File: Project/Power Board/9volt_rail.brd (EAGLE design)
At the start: 98.3 x 69.5 mm, 54 parts, among them IC1 TL331, Q1 BSS84, Q2 BSS123

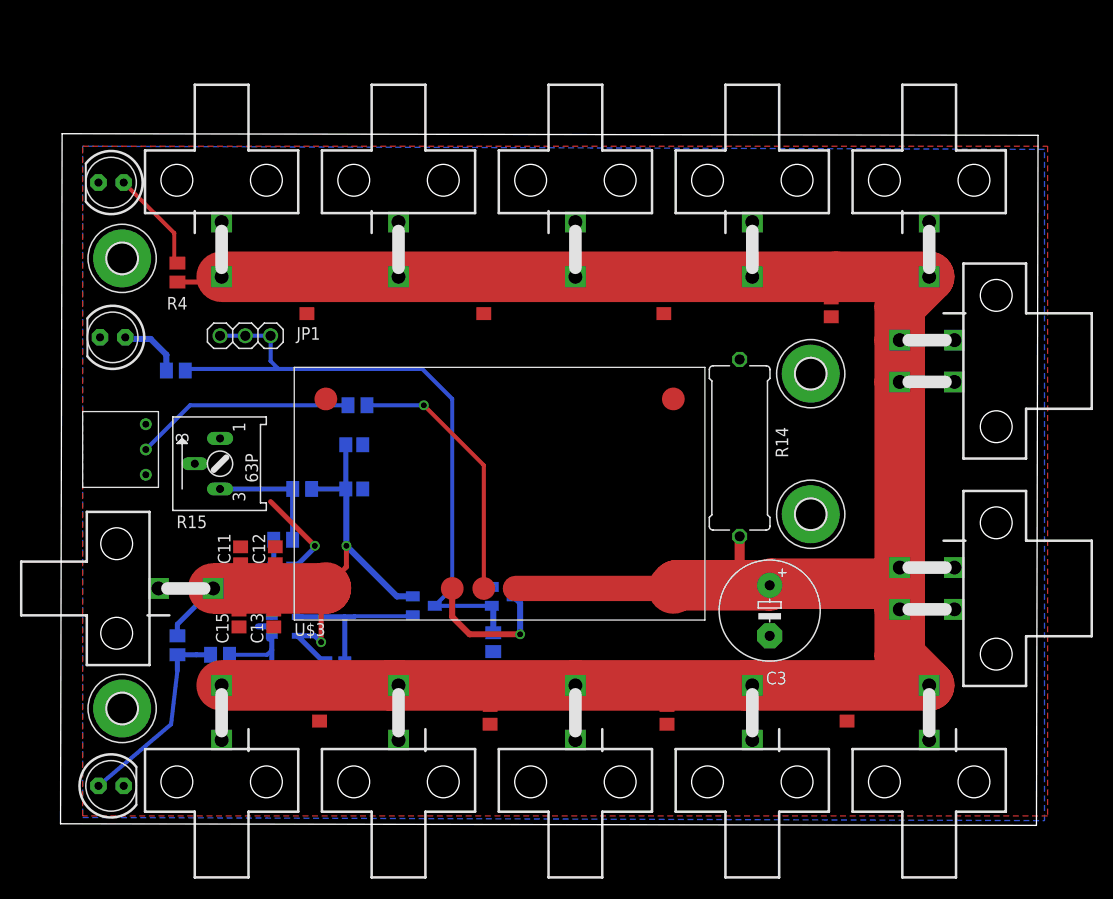
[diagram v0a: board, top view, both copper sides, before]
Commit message: update
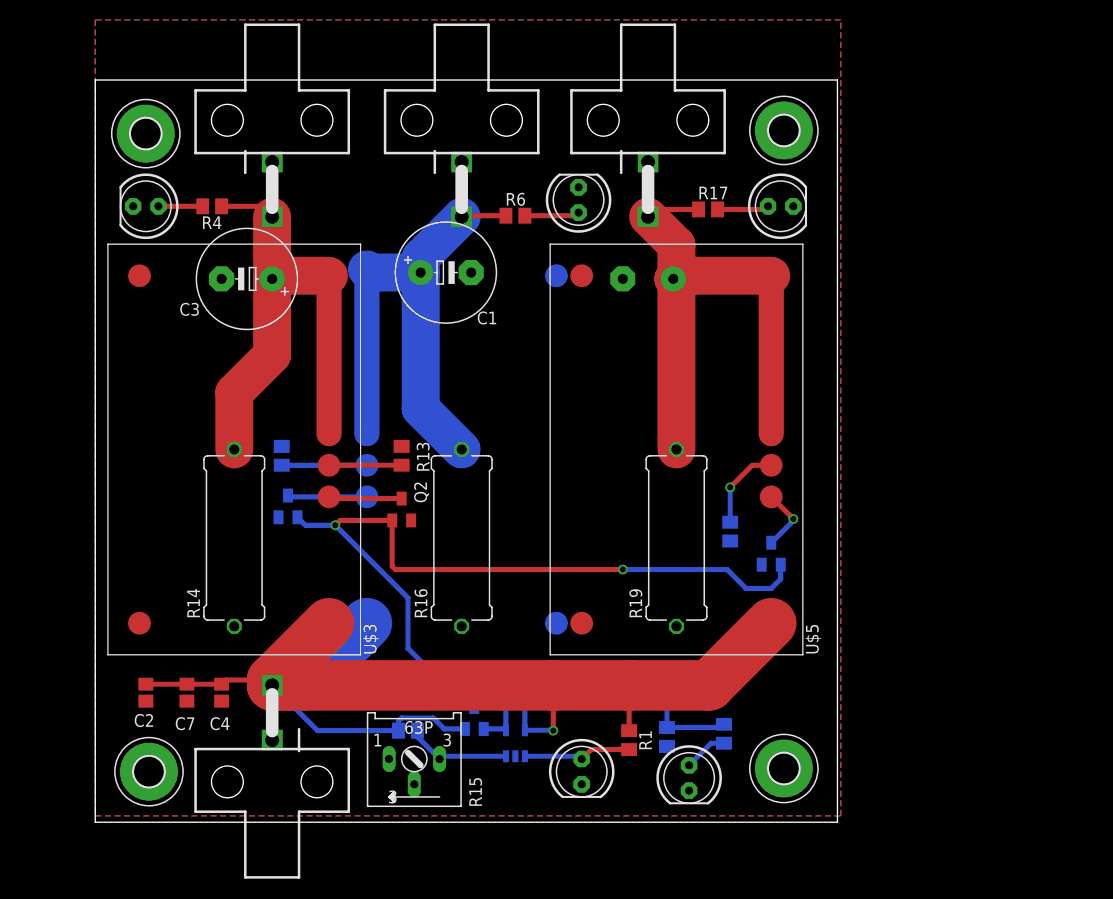
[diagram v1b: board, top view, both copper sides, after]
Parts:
- removed C10, C5, C8, C9: (no value), rcl:C0805
- removed C11, C12, C13, C14, C15: 2.2uF, adafruit:C0805
- removed JP1: (no value), adafruit:1X03
- removed PL10, PL3, PL5, PL6, PL7, PL8, PL9: (no value), con-molex-2:5569-2
- removed PL11, PL13: (no value), con-molex-2:5569-4
- removed R2, R5, R7, R9: (no value), adafruit:M0805
- removed U$4: 3310-001, 3310-001:3310-001-TH
- added Q3, Q4: BSS123, transistor-small-signal:SOT23
- added R10, R17, R18, R6: (no value), adafruit:M0805
- added R16, R19: (no value), resistor:0617/17
- added U$1, U$5: PTH78020-SMD, PTN78020:PTN78020-SND
- added VCC4, VCC5: (no value), adafruit:LED5MM
- C1, C6: value (none) -> 330uF; device rcl:C0805 -> rcl:E5-10,5
- C2, C7: value (none) -> 2.2uF; device rcl:C0805 -> adafruit:C0805
- moved H4 77.6 mm to (5.40, 4.45)
- moved PL4 75.5 mm to (17.8, 65.7), turned to 180 degrees
- moved VCC3 72.9 mm to (59.7, 3.81), turned to 270 degrees
- moved H2 67.7 mm to (69.2, 68.9)
- moved R11 66.1 mm to (63.2, 8.26), turned to 270 degrees
- moved C2 65.1 mm to (5.08, 12.4), turned to 270 degrees
- moved PL2 63.3 mm to (55.6, 65.7), turned to 180 degrees
- moved PL1 62.9 mm to (36.8, 65.7), turned to 180 degrees
- moved C3 62.2 mm to (15.2, 54.0), turned to 180 degrees
- moved H3 57.8 mm to (5.08, 68.6)
- moved R14 51.6 mm to (14.0, 27.9), turned to 90 degrees
- moved C6 47.9 mm to (55.6, 54.0), flipped to the bottom, turned to 0 degrees
- moved VCC1 47.3 mm to (48.9, 4.45), turned to 270 degrees
- moved R1 46.4 mm to (53.7, 7.62), flipped to the top
- moved R15 35.5 mm to (32.1, 5.71), turned to 180 degrees
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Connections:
- removed net N$1: R13.2, U$4.2
- removed net N$3: R1.2, R5.1, VCC1.A
- removed net N$5: JP1.1, JP1.2, JP1.3, Q1.3, Q2.1, R11.1, R12.1
- removed net N$6: R15.E, R2.1, R3.2
- new net N$14: R6.2, VCC4.A
- new net N$15: C1.+, PL1.2, R16.2, R6.1, U$1.5, U$1.6
- new net N$16: R10.1, U$1.4
- new net N$18: Q3.3, U$1.3
- new net N$19: R17.2, VCC5.A
- new net N$20: C6.+, PL2.2, R17.1, R19.2, U$5.5, U$5.6
- new net N$21: R18.1, U$5.4
- new net N$23: Q4.3, U$5.3
- new net N$24: Q1.3, Q2.1, Q3.1, Q4.1, R11.1, R12.1
- net GND: now also C1.-, C2.2, C6.-, C7.2, Q3.2, Q4.2, R10.2, R13.2, R16.1, R18.2, R19.1, U$1.1, U$1.7, U$5.1, U$5.7, VCC4.K, VCC5.K; no longer C1.1, C10.1, C11.2, C12.2, C13.2, C14.2, C15.2, C2.1, C5.1, C6.1, C7.1, C8.1, C9.1, PL10.1, PL11.1, PL11.2, PL13.1, PL13.2, PL3.1, PL5.1, PL6.1, PL7.1, PL8.1, PL9.1, R7.2, U$4.3
- net N$11: no longer C1.2, C10.2, C2.2, C5.2, C6.2, C7.2, C8.2, C9.2, PL1.2, PL10.2, PL11.3, PL11.4, PL13.3, PL13.4, PL2.2, PL3.2, PL5.2, PL6.2, PL7.2, PL8.2, PL9.2
- net N$2: no longer R9.2
- net N$4: now also R15.E, R3.2; no longer R2.2, R9.1
- net N$7: now also R1.2, VCC1.A; no longer R5.2, R7.1
- net VCC: now also C2.1, C7.1, U$1.2, U$5.2; no longer C11.1, C12.1, C13.1, C14.1, C15.1
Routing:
- net N$11: track 304.0 -> 53.6 mm
- net N$24: track 0.00 -> 117.3 mm, vias 0 -> 2
- net N$5: track 66.9 -> 0.00 mm
- net N$20: track 0.00 -> 55.6 mm
- net N$15: track 0.00 -> 53.3 mm
- net VCC: track 78.4 -> 124.3 mm, vias 2 -> 1
- net N$2: track 31.4 -> 6.05 mm, vias 1 -> 0
- net N$1: track 22.4 -> 0.00 mm
- net N$3: track 19.9 -> 0.00 mm
- net N$13: track 26.6 -> 7.30 mm, vias 1 -> 0
- net N$6: track 12.4 -> 0.00 mm
- net N$16: track 0.00 -> 8.57 mm
- net N$21: track 0.00 -> 8.54 mm, vias 0 -> 1
- net N$18: track 0.00 -> 8.00 mm
- net N$10: track 14.5 -> 7.37 mm, vias 1 -> 0
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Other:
- board size 98.3 x 69.5 mm -> 74.6 x 74.6 mm
